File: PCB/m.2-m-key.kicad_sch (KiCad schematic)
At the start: 16 parts, among them J1 M.2 M-Key Edge Connector

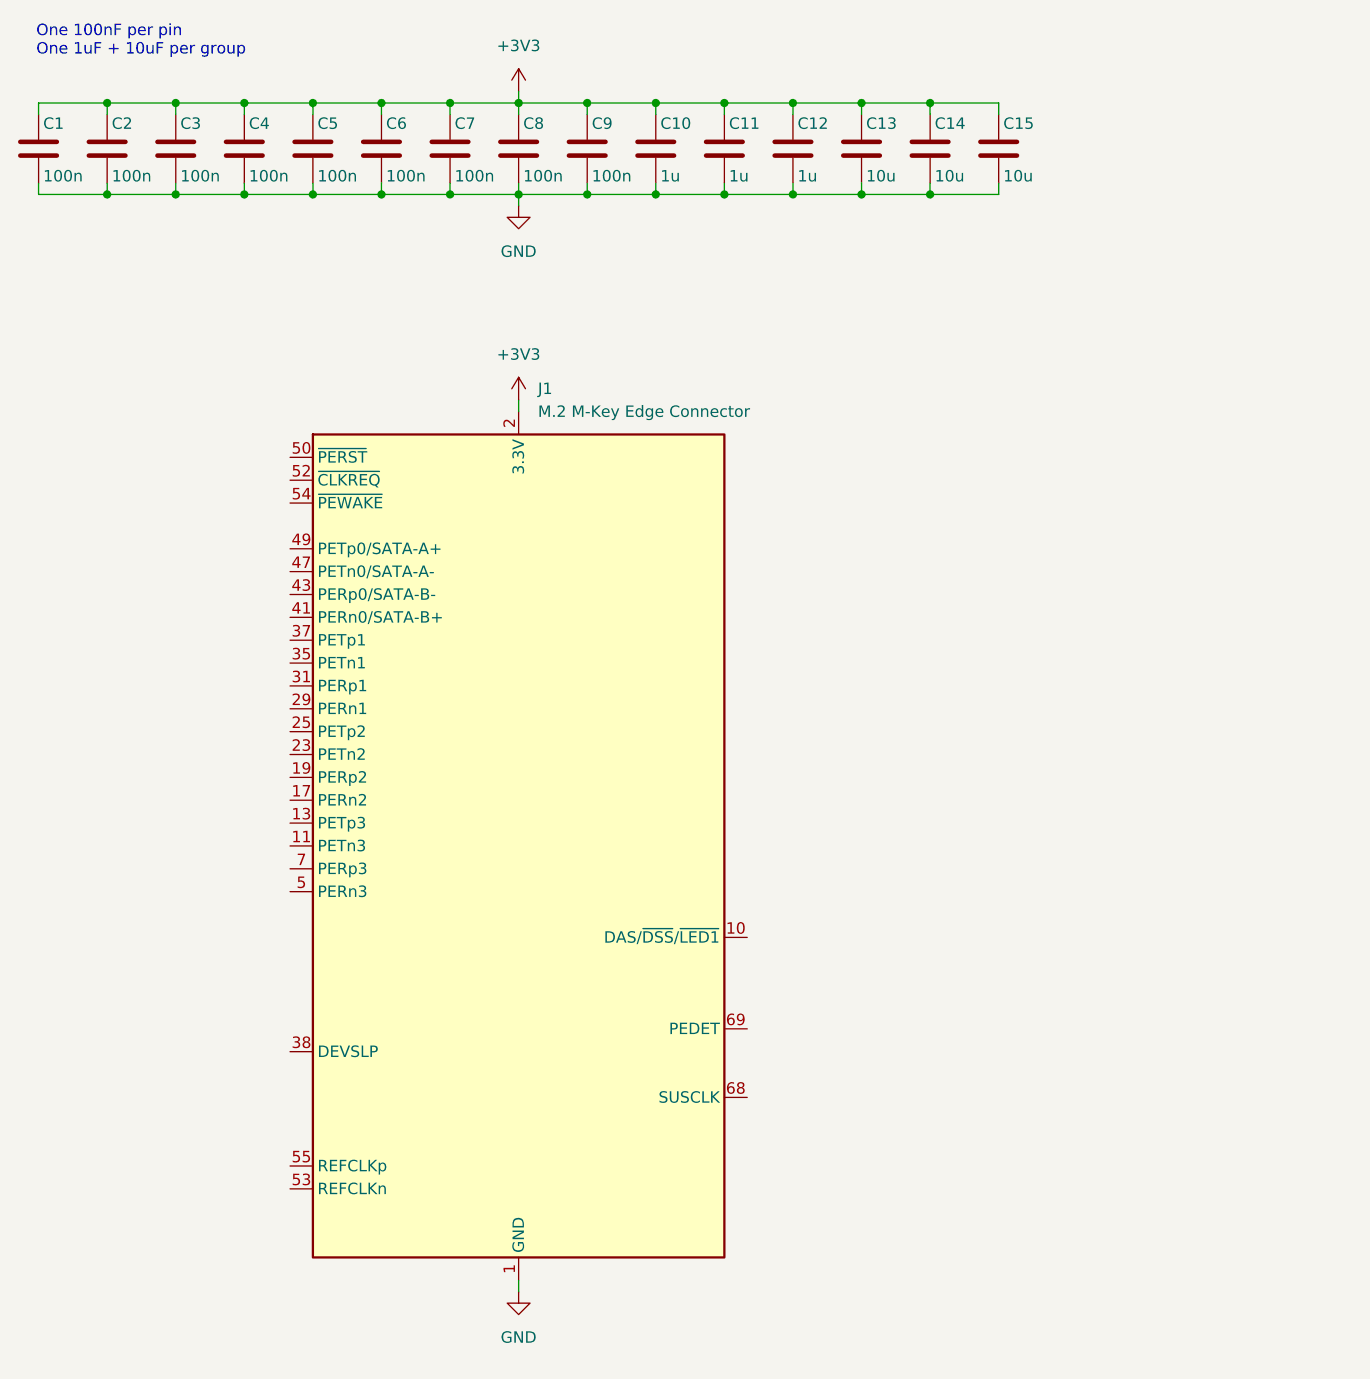
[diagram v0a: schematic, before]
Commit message: cleaning up the schematic some more
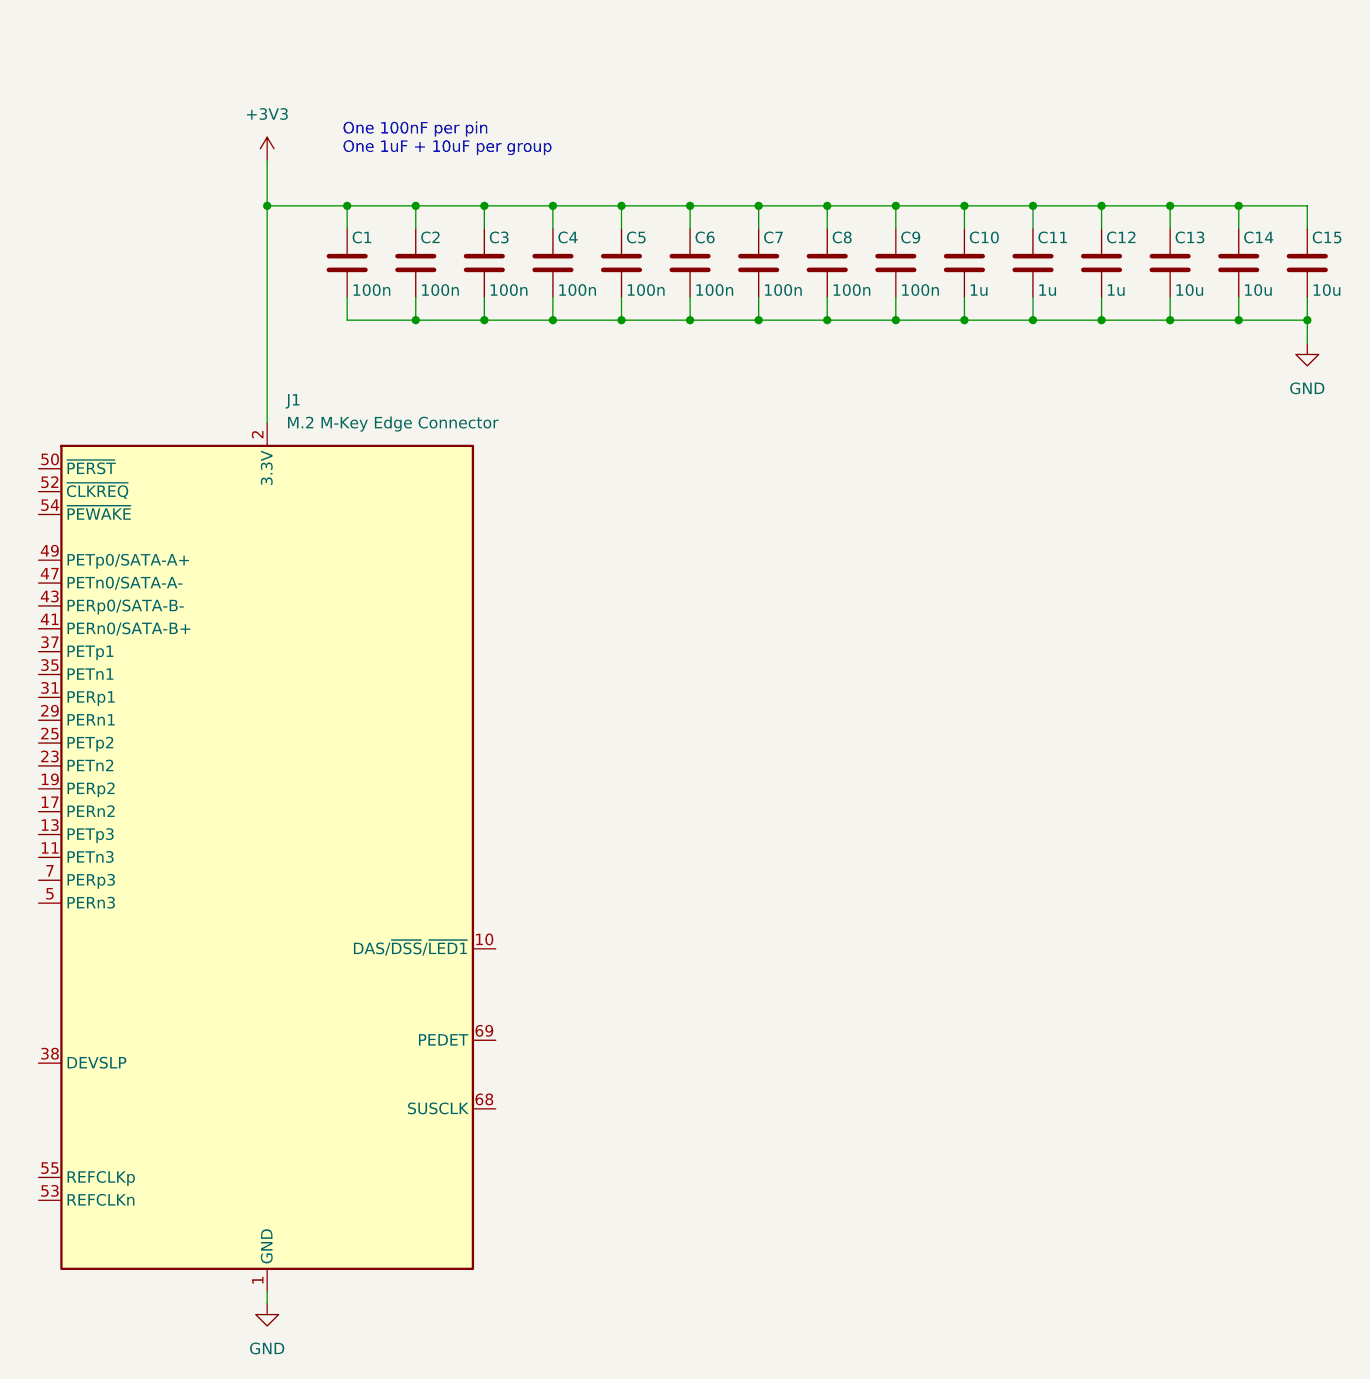
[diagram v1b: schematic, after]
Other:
- moved on the sheet: C10, C11, C12, C13, C14, C15, C2, C3, C4, C5, C6, C7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
